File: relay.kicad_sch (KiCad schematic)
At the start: 19 parts, among them J10 Signal Relay A/B 1, J11 Signal Relay A/B 2, J6 Power Relay 0, J7 Power Relay 1, J8 Power Relay 2, J9 Signal Relay A/B 0, K1 G5LE-1, K2 G5LE-1, K3 G5LE-1, K4 G6K-2, K5 G6K-2, K6 G6K-2, U2 ULN2803A

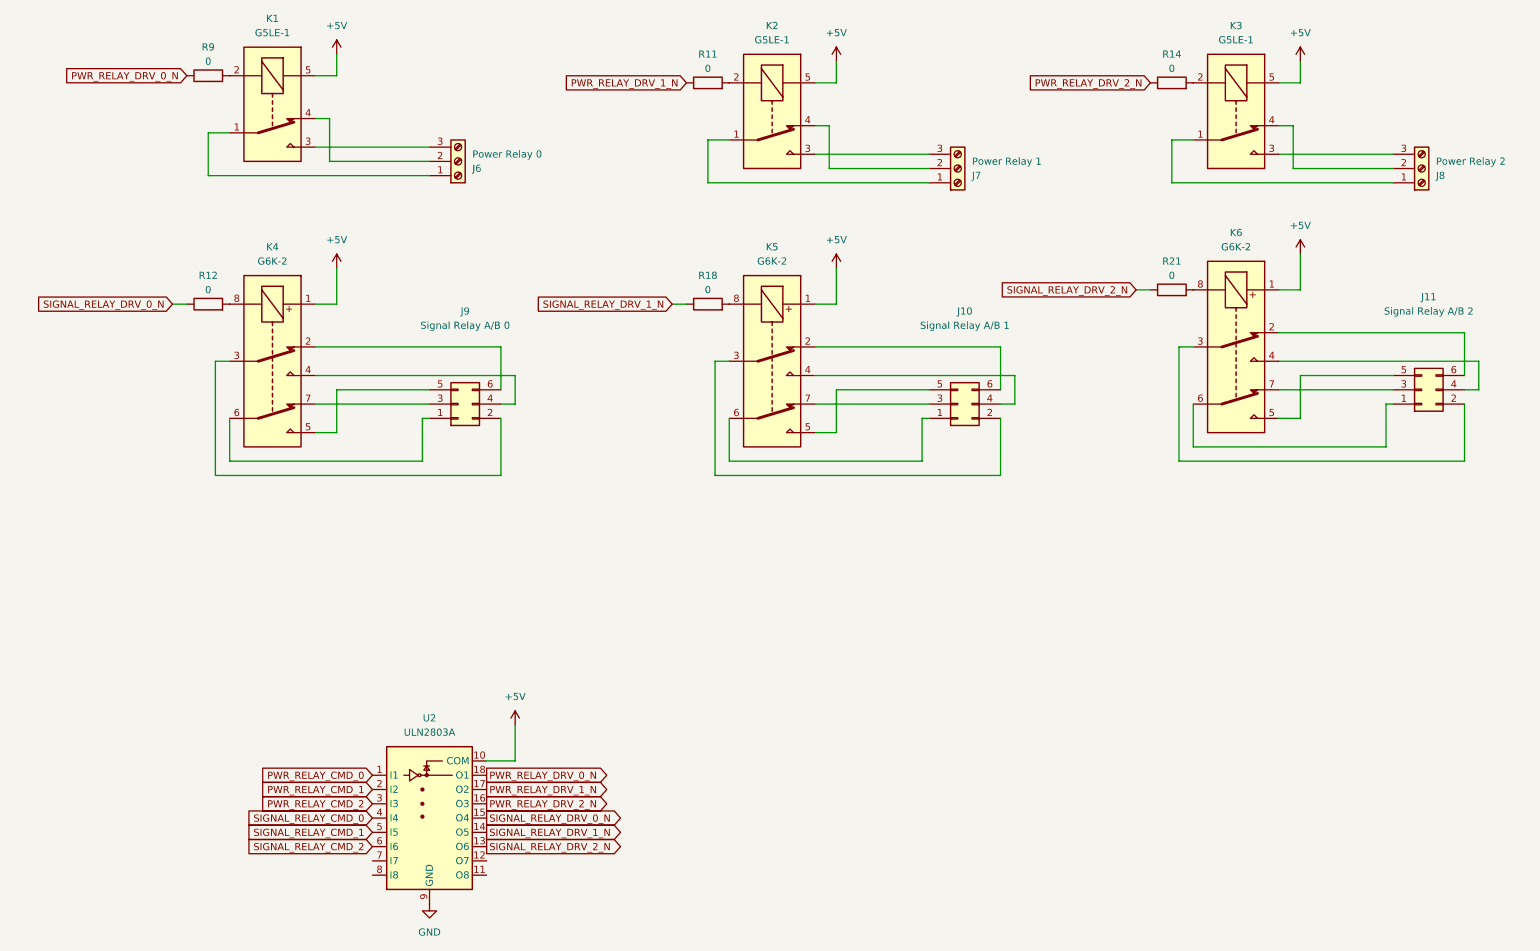
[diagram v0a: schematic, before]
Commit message: session 5
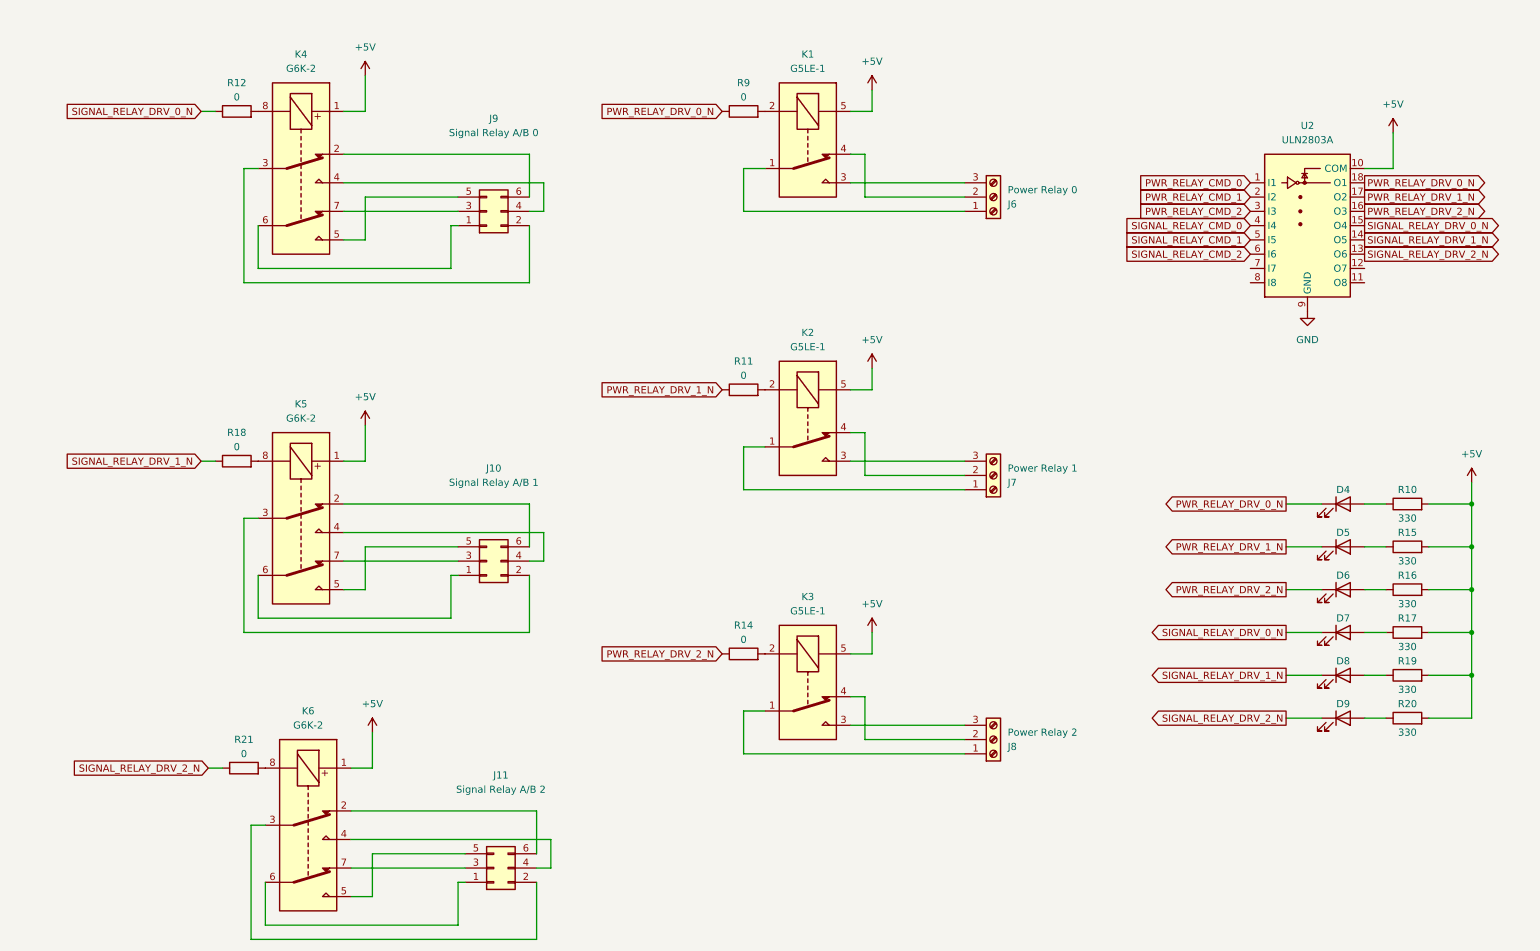
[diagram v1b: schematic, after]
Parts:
- added D4, D5, D6, D7, D8, D9: LED, symbol Device:LED
- added R10, R15, R16, R17, R19, R20: 330, symbol Device:R
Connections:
- net +5V: now also R10.2, R15.2, R16.2, R17.2, R19.2, R20.2
- net PWR_RELAY_DRV_0_N: now also D4.1 (K)
- net PWR_RELAY_DRV_1_N: now also D5.1 (K)
- net PWR_RELAY_DRV_2_N: now also D6.1 (K)
- net SIGNAL_RELAY_DRV_0_N: now also D7.1 (K)
- net SIGNAL_RELAY_DRV_1_N: now also D8.1 (K)
- net SIGNAL_RELAY_DRV_2_N: now also D9.1 (K)
- new net: D7.2 (A), R17.1
- new net: D6.2 (A), R16.1
- new net: D4.2 (A), R10.1
- new net: D5.2 (A), R15.1
- new net: D9.2 (A), R20.1
- new net: D8.2 (A), R19.1
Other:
- moved on the sheet: J10, J11, J6, J7, J8, J9, K1, K2, K3, K4, K5, K6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
